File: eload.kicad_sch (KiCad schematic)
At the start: 23 parts, among them J1 Device Power, J2 Input Power, J3 SWD Header, Q1 TIP122, SW1 RotaryEncoder_Switch, U1 STM32F103C8T6, U2 LM1117DT-3.3, U3 AD8629, U4 MCP4725

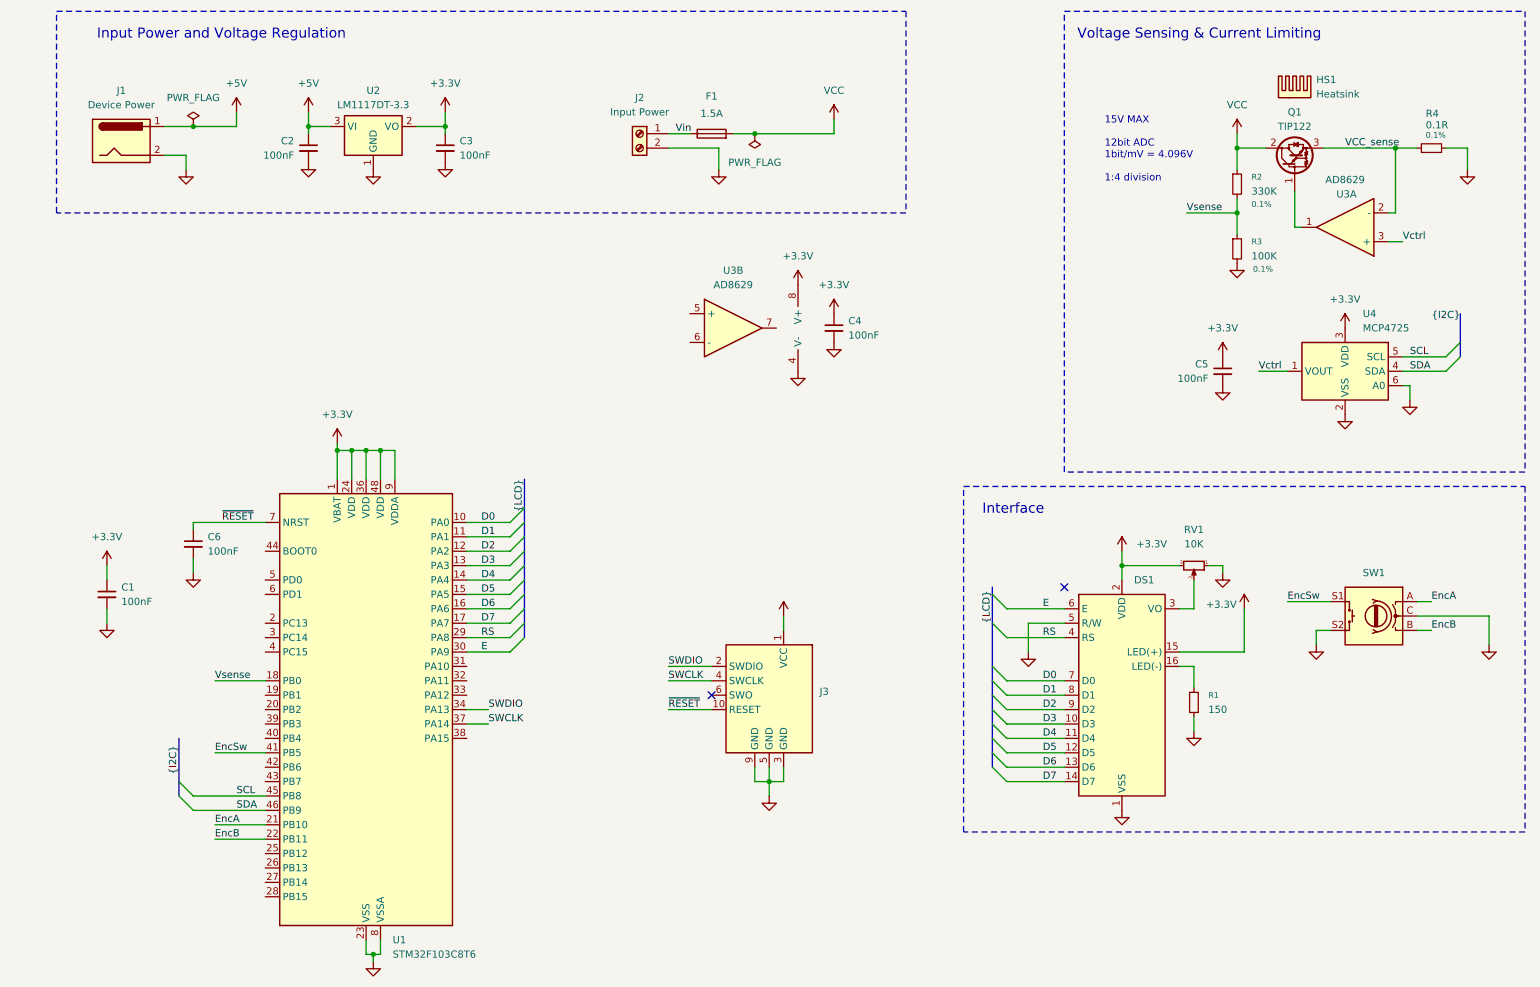
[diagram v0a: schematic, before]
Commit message: WIP schematic
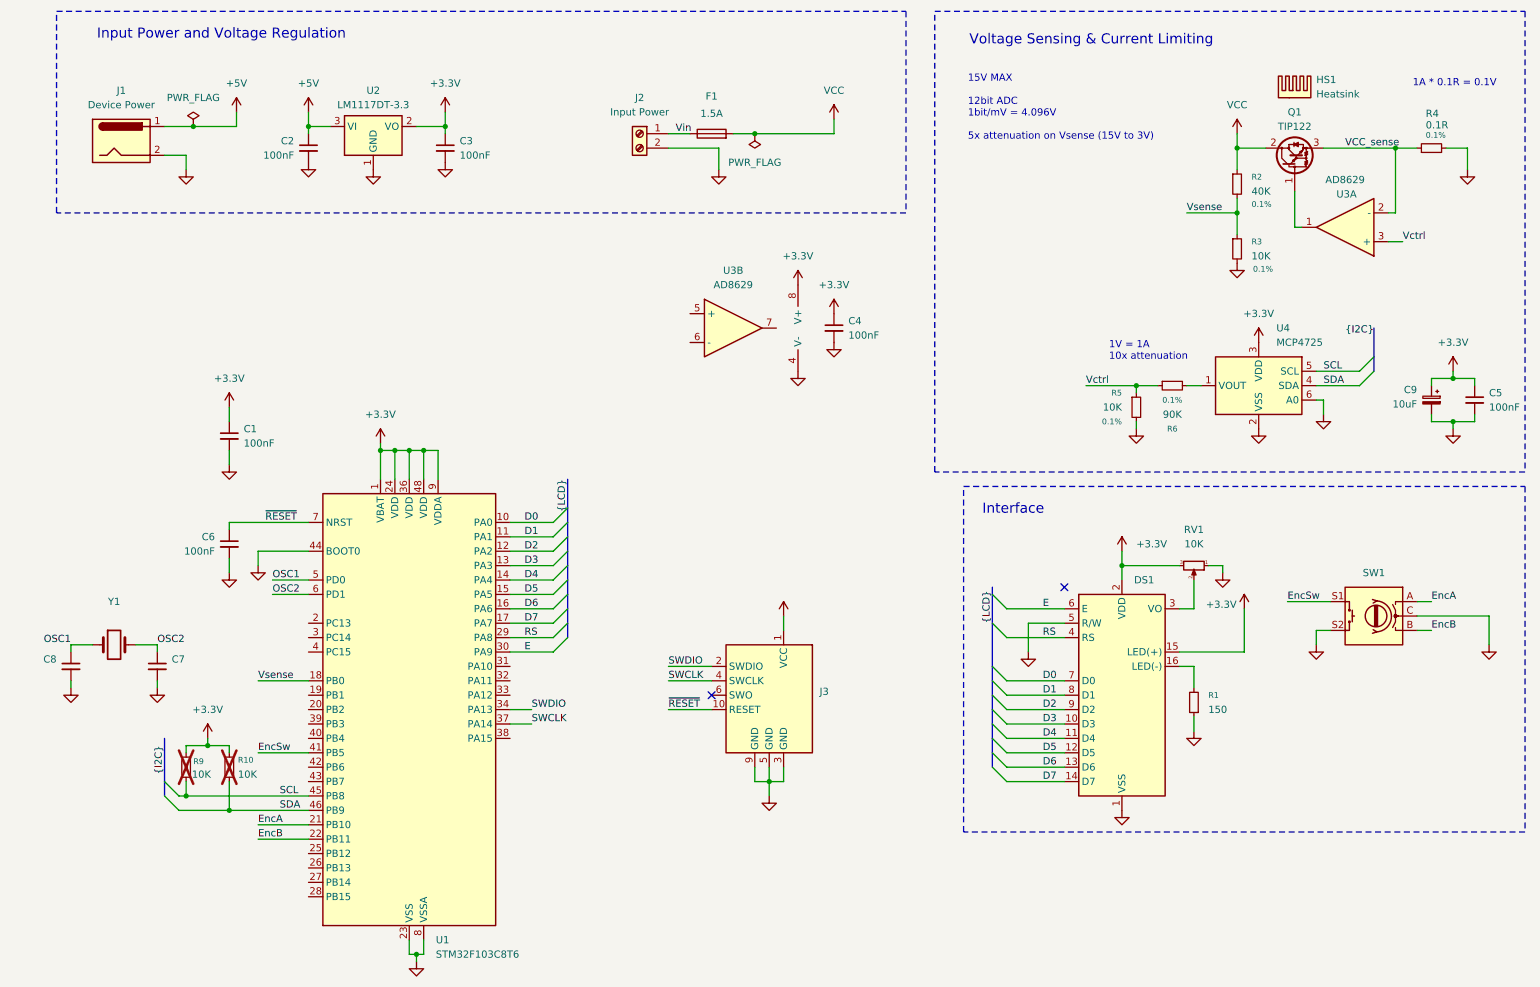
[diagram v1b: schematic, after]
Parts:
- added C7, C8: C_Small, symbol Device:C_Small
- added C9: 10uF, symbol Device:C_Polarized_Small
- added R10, R5, R9: 10K, symbol Device:R_Small
- added R6: 90K, symbol Device:R_Small
- added Y1: Crystal, symbol Device:Crystal
- R2: value 330K -> 40K
- R3: value 100K -> 10K
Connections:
- net +3.3V: now also C9.1, R10.1, R9.1
- net GND: now also U1.44 (BOOT0), C7.2, C8.2, C9.2, R5.2
- net SCL: now also R9.2
- net SDA: now also R10.2
- net Vctrl: now also R5.1, R6.1; no longer U4.1 (VOUT)
- net OSC1: now reaches U1.5 (PD0)
- net OSC1: now also C8.1, Y1.1
- net OSC2: now reaches U1.6 (PD1)
- net OSC2: now also C7.1, Y1.2
- new net: R6.2, U4.1 (VOUT)
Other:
- note added: "15V MAX 12bit ADC 1bit/mV = 4.096V 5x attenuation on Vsense (15V to 3V)"
- note added: "1A * 0.1R = 0.1V"
- note added: "1V = 1A 10x attenuation"
- note removed: "15V MAX 12bit ADC 1bit/mV = 4.096V 1:4 division"
- moved on the sheet: C1, C5, C6, U1, U4
